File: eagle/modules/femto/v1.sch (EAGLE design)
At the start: 50 parts, among them IC1 MEGA8-AI, J1 RJ12RIGHTANGLE-I2C, J2 RJ12RIGHTANGLE-I2C

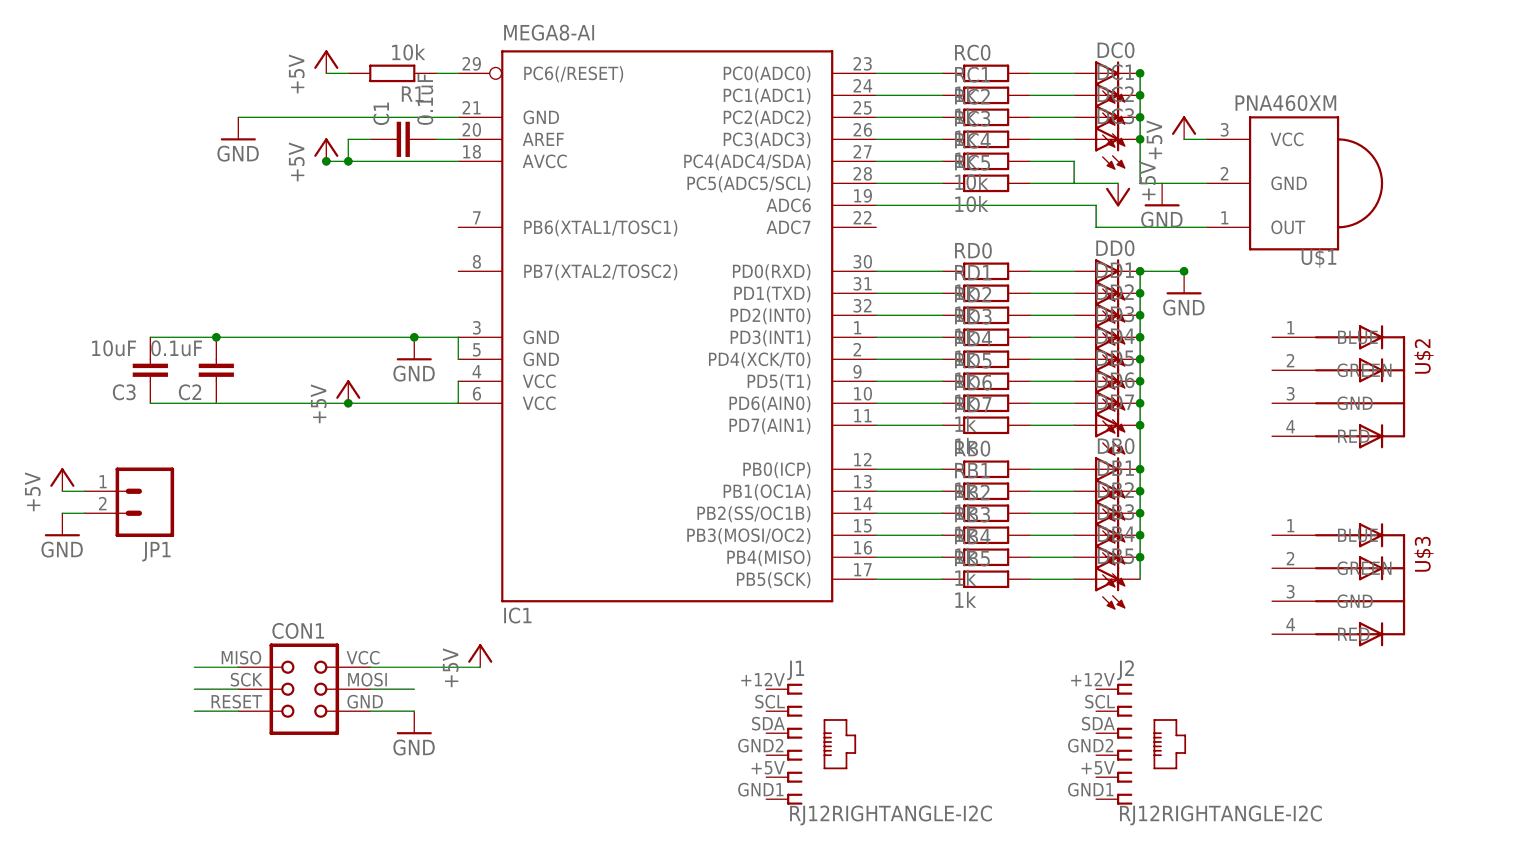
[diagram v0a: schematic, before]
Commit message: Update femto
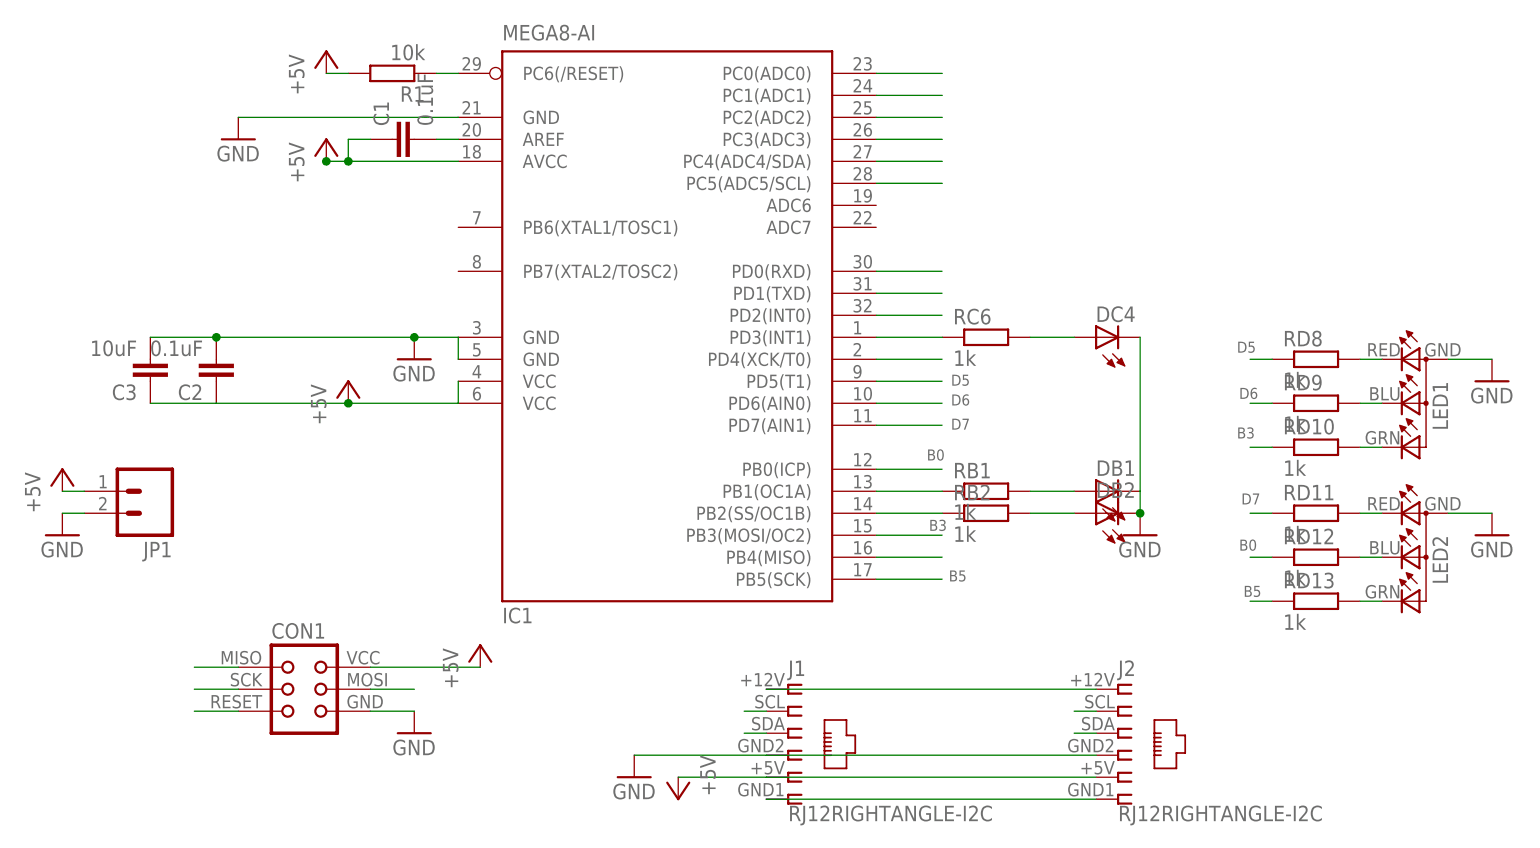
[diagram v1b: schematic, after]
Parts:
- removed DB0, DB3, DB4, DB5, DC0, DC1, DC2, DC3, DD0, DD1, DD2, DD4, DD5, DD6, DD7: (no value), led:LED3MM
- removed RB0, RB3, RB4, RB5, RC0, RC1, RC2, RC3, RD0, RD1, RD2, RD4, RD5, RD6, RD7: 1k, resistor:R-EU_M1206
- removed RC4, RC5: 10k, resistor:R-EU_M1206
- removed U$1: PNA460XM, adafruit:PNA460XM
- removed U$2, U$3: 5MMRGBLED, adafruit:5MMRGBLED
- added LED1, LED2: (no value), lpatiny:TOPLED-3
- added RD10, RD11, RD12, RD13, RD8, RD9: 1k, resistor:R-EU_M1206
- renumbered DD3 to DC4, RD3 to RC6
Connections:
- removed net N$15: IC1.PD6(AIN0), RD6.1
- removed net N$16: IC1.PD7(AIN1), RD7.1
- removed net N$25: DC0.A, RC0.2
- removed net N$26: DC1.A, RC1.2
- removed net N$27: DC2.A, RC2.2
- removed net N$28: DC3.A, RC3.2
- removed net N$31: DD0.A, RD0.2
- removed net N$32: DD1.A, RD1.2
- removed net N$33: DD2.A, RD2.2
- removed net N$35: DD4.A, RD4.2
- removed net N$36: DD5.A, RD5.2
- removed net N$37: DD6.A, RD6.2
- removed net N$38: DD7.A, RD7.2
- removed net N$39: DB0.A, RB0.2
- removed net N$42: DB3.A, RB3.2
- removed net N$43: DB4.A, RB4.2
- removed net N$46: DB5.A, RB5.2
- removed net N$47: IC1.ADC6, U$1.OUT
- new net B0: IC1.PB0(ICP), RD12.1
- new net B3: IC1.PB3(MOSI/OC2), RD10.1
- new net B5: IC1.PB5(SCK), RD13.1
- new net D5: IC1.PD5(T1), RD8.1
- new net D6: IC1.PD6(AIN0), RD9.1
- new net D7: IC1.PD7(AIN1), RD11.1
- new net N$1: LED1.CRED, RD8.2
- new net N$20: LED2.CRED, RD11.2
- new net N$21: LED2.CBLUE, RD12.2
- new net N$22: LED2.CGREEN, RD13.2
- new net N$7: LED1.CBLUE, RD9.2
- new net N$8: LED1.CGREEN, RD10.2
- net +5V: now also J1.5, J2.5; no longer RC4.2, RC5.2, U$1.VCC
- net GND: now also J1.4, J2.4, LED1.A2, LED2.A2; no longer DB0.C, DB3.C, DB4.C, DB5.C, DC0.C, DC1.C, DC2.C, DC3.C, DD0.C, DD1.C, DD2.C, DD4.C, DD5.C, DD6.C, DD7.C, U$1.GND
- net MISO: no longer RB4.1
- net MOSI: no longer IC1.PB3(MOSI/OC2), RB3.1
- net N$10: no longer RD1.1
- net N$12: no longer RD2.1
- net N$13: now also J1.1, J2.1; no longer IC1.PD5(T1), RD5.1
- net N$14: no longer RD4.1
- net N$17: now also J1.6, J2.6; no longer IC1.PB0(ICP), RB0.1
- net N$2: no longer RC1.1
- net N$3: no longer RC0.1
- net N$5: no longer RC3.1
- net N$6: no longer RC2.1
- net N$9: no longer RD0.1
- net SCK: no longer IC1.PB5(SCK), RB5.1
- net SCL: now also J1.2, J2.2; no longer RC5.1
- net SDA: now also J1.3, J2.3; no longer RC4.1
